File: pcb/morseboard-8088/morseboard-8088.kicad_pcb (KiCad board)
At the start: 2 copper layers, 161 x 108 mm, 65 parts, among them J1 USB_B, J2 UART1, J3 TxD, J4 ~{CTS}, J5 RxD, J6 ~{RTS}, SW1 SW_SPDT, SW2 INTPORT, SW4 NMI, SW6 RESET, U1 8088, U10 74HCT273, U11 TL16C550, U12 74HC245, U13 MAX232, U14 DS1813, U2 74HCT573, U3 74HCT573, U4 74HCT245, U5 SST39SF040, U6 74HCT138, U7 74HCT02, U8 74HCT00, U9 AS6C4008-55PCN, X1 7.3728 MHz

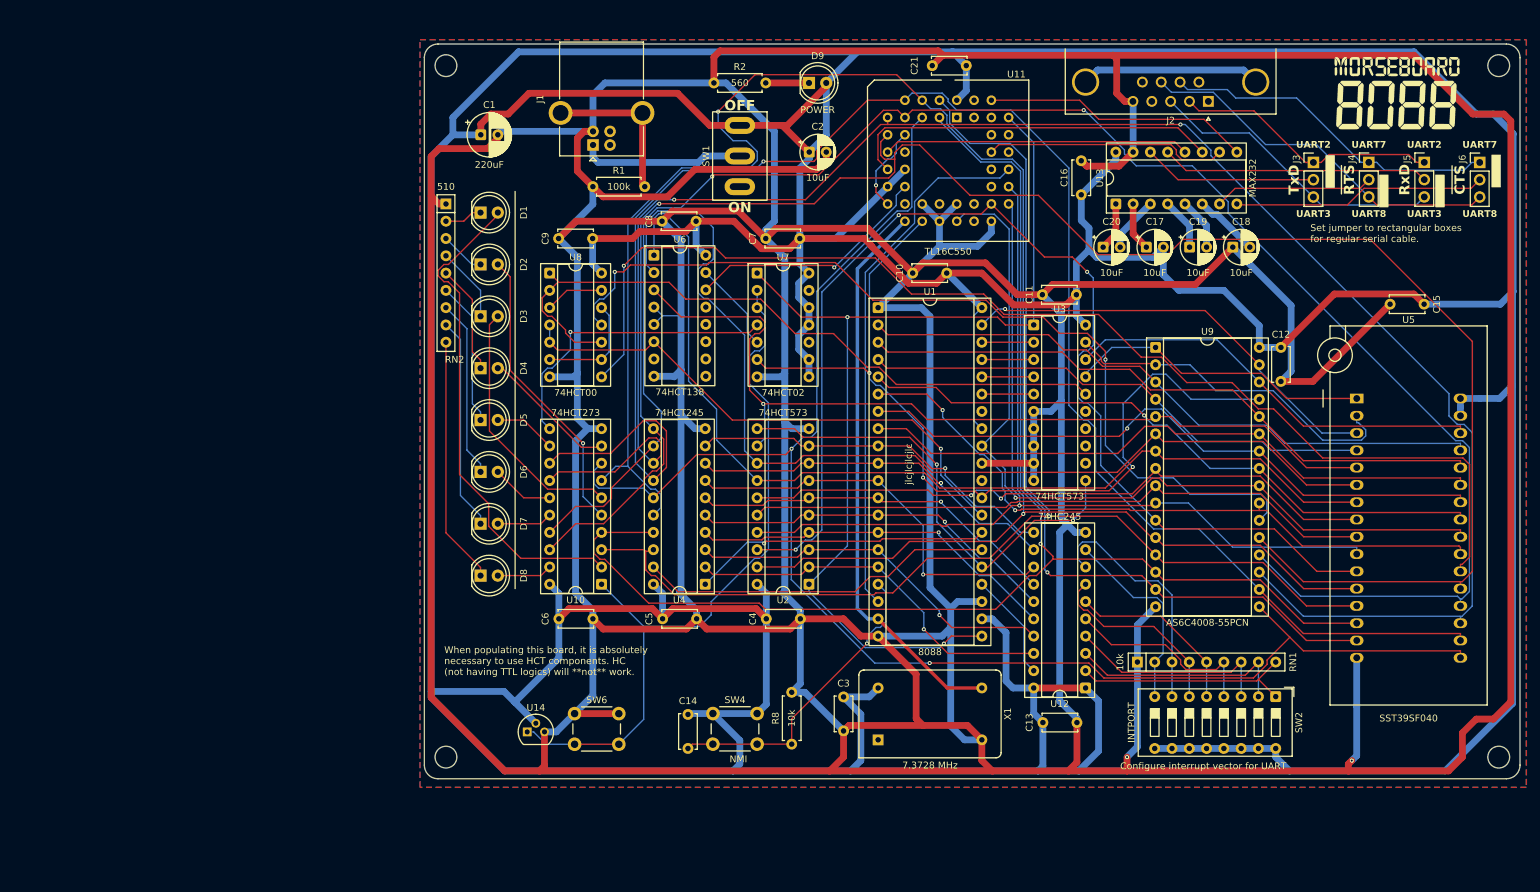
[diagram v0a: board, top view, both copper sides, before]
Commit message: Fixing bugs in PCB design
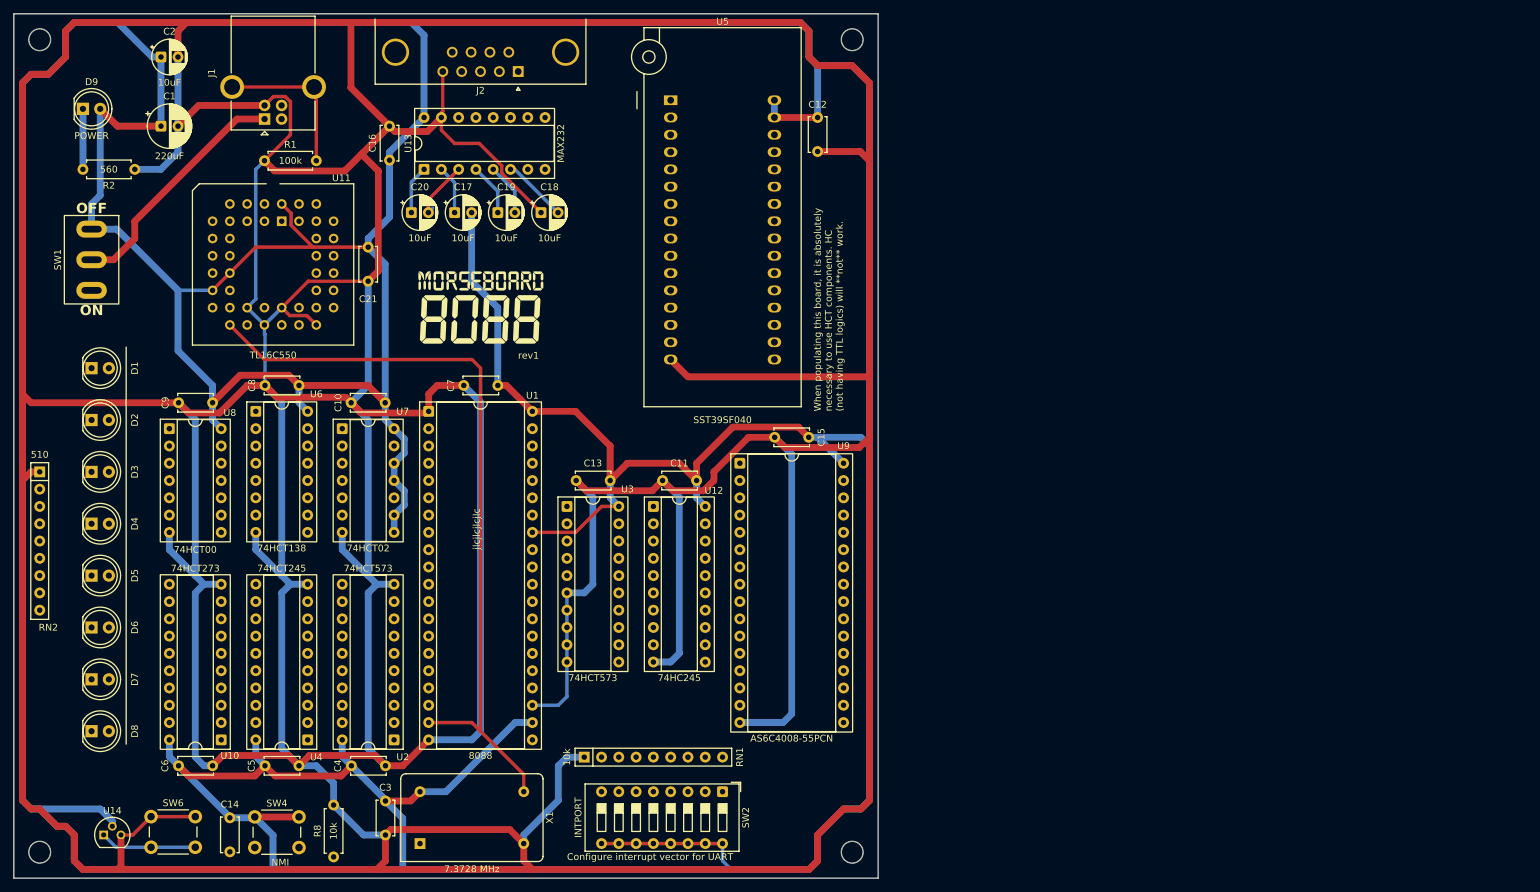
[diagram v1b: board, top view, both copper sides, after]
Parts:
- removed J3: TxD, Connector_PinHeader_2.54mm:PinHeader_1x03_P2.54mm_Vertical
- removed J4: ~{CTS}, Connector_PinHeader_2.54mm:PinHeader_1x03_P2.54mm_Vertical
- removed J5: RxD, Connector_PinHeader_2.54mm:PinHeader_1x03_P2.54mm_Vertical
- removed J6: ~{RTS}, Connector_PinHeader_2.54mm:PinHeader_1x03_P2.54mm_Vertical
- moved G*** 138.3 mm to (88.9, 63.5)
- moved U5 109.9 mm to (116.8, 33.0)
- moved D9 106.7 mm to (30.5, 34.3)
- moved C19 101.8 mm to (91.4, 49.5)
- moved C18 101.8 mm to (97.8, 49.5)
- moved C20 101.8 mm to (78.7, 49.5)
- moved U13 101.8 mm to (80.6, 43.2)
- moved C16 101.8 mm to (75.5, 41.8)
- moved C17 101.8 mm to (85.1, 49.5)
- moved J2 101.5 mm to (94.4, 28.8)
- moved U11 100.4 mm to (59.7, 50.8)
- moved SW1 96.5 mm to (31.8, 56.5)
- moved C2 96.3 mm to (42.0, 26.7)
- moved H4 96.0 mm to (143.5, 143.5)
- moved H2 95.1 mm to (143.5, 24.1)
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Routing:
- net D7: track 276.9 -> 0.00 mm, vias 1 -> 0
- net D5: track 271.1 -> 0.00 mm, vias 2 -> 0
- net D6: track 263.0 -> 0.00 mm, vias 2 -> 0
- net D4: track 255.8 -> 0.00 mm, vias 1 -> 0
- net D2: track 248.0 -> 0.00 mm, vias 2 -> 0
- net D3: track 229.2 -> 0.00 mm, vias 2 -> 0
- net D1: track 208.1 -> 0.00 mm, vias 1 -> 0
- net D0: track 198.0 -> 0.00 mm, vias 1 -> 0
- net ~{ROMCS}: track 172.6 -> 0.00 mm, vias 1 -> 0
- net A1: track 170.1 -> 0.00 mm, vias 3 -> 0
- net A6: track 154.3 -> 0.00 mm
- net RES: track 148.0 -> 0.00 mm, vias 2 -> 0
- net A5: track 147.0 -> 0.00 mm
- net A0: track 145.1 -> 0.00 mm, vias 1 -> 0
- net A2: track 138.8 -> 0.00 mm, vias 1 -> 0
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- removed copper zone on F.Cu, net GND
- removed copper zone on B.Cu, net VCC
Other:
- board size 161 x 108 mm -> 127 x 127 mm
- board text added: "rev1"
- board text removed: "RxD"
- board text removed: "Set jumper to rectangular boxes for regular serial cable."
- board text removed: "TxD"
- board text removed: "UART2"
- board text removed: "UART3"
- board text removed: "UART7"
- board text removed: "UART8"
- board text removed: "~{CTS}"
- board text removed: "~{RTS}"
